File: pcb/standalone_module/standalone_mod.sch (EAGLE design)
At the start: 11 parts, among them U1 V_REG_317DPACK

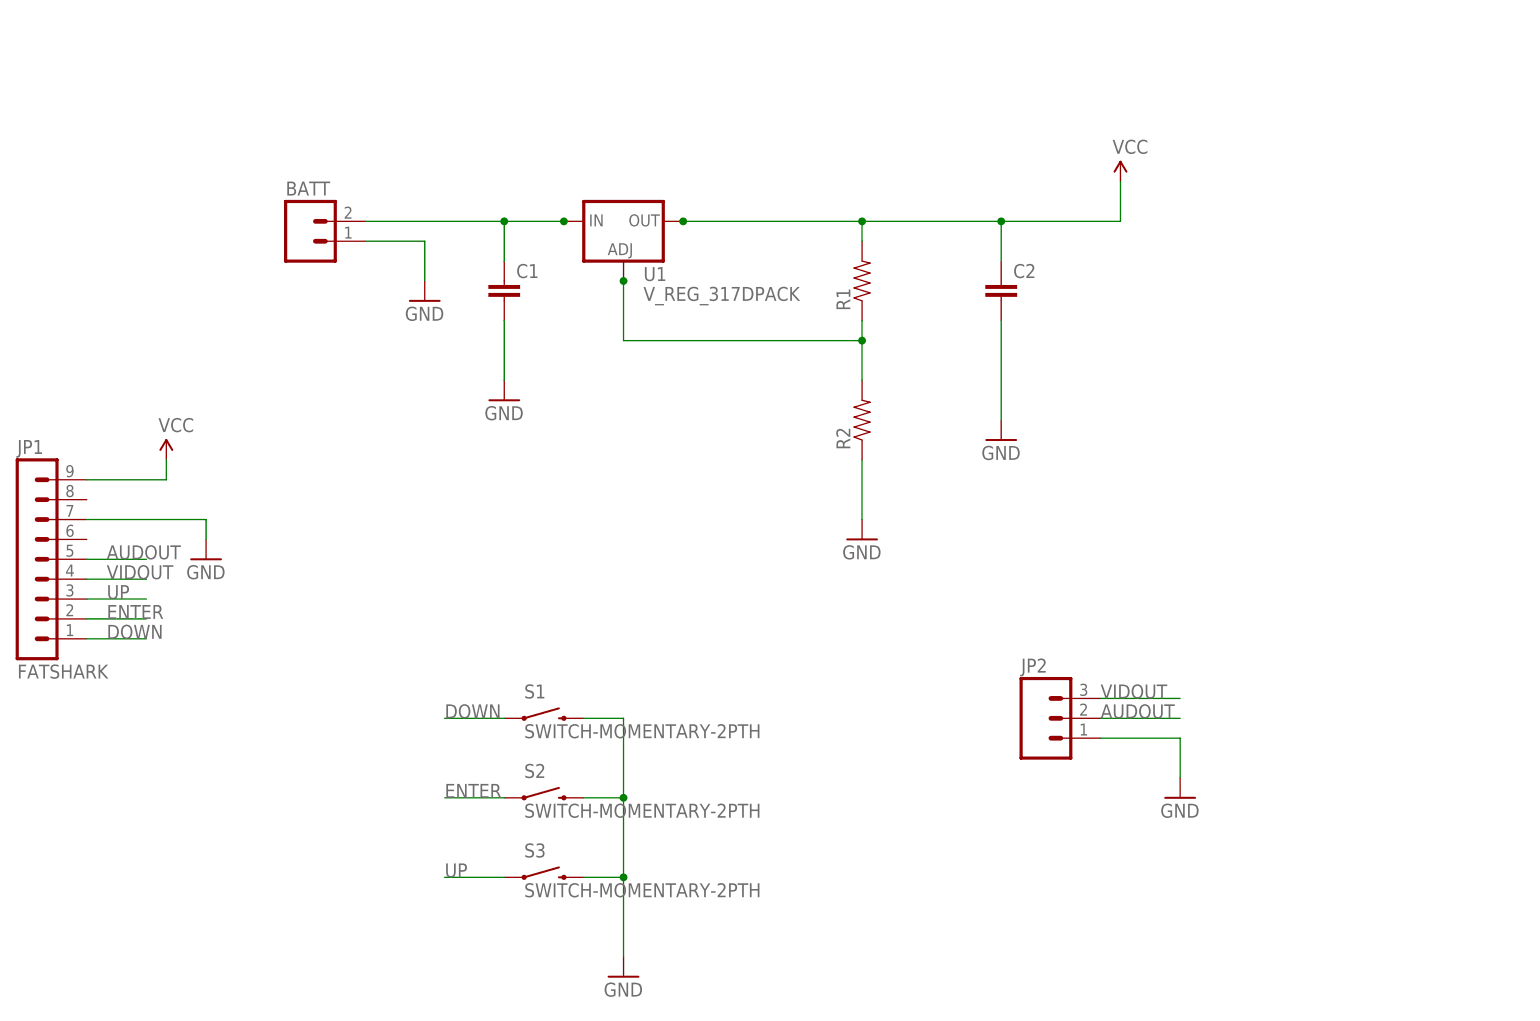
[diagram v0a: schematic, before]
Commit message: standalone v2.0
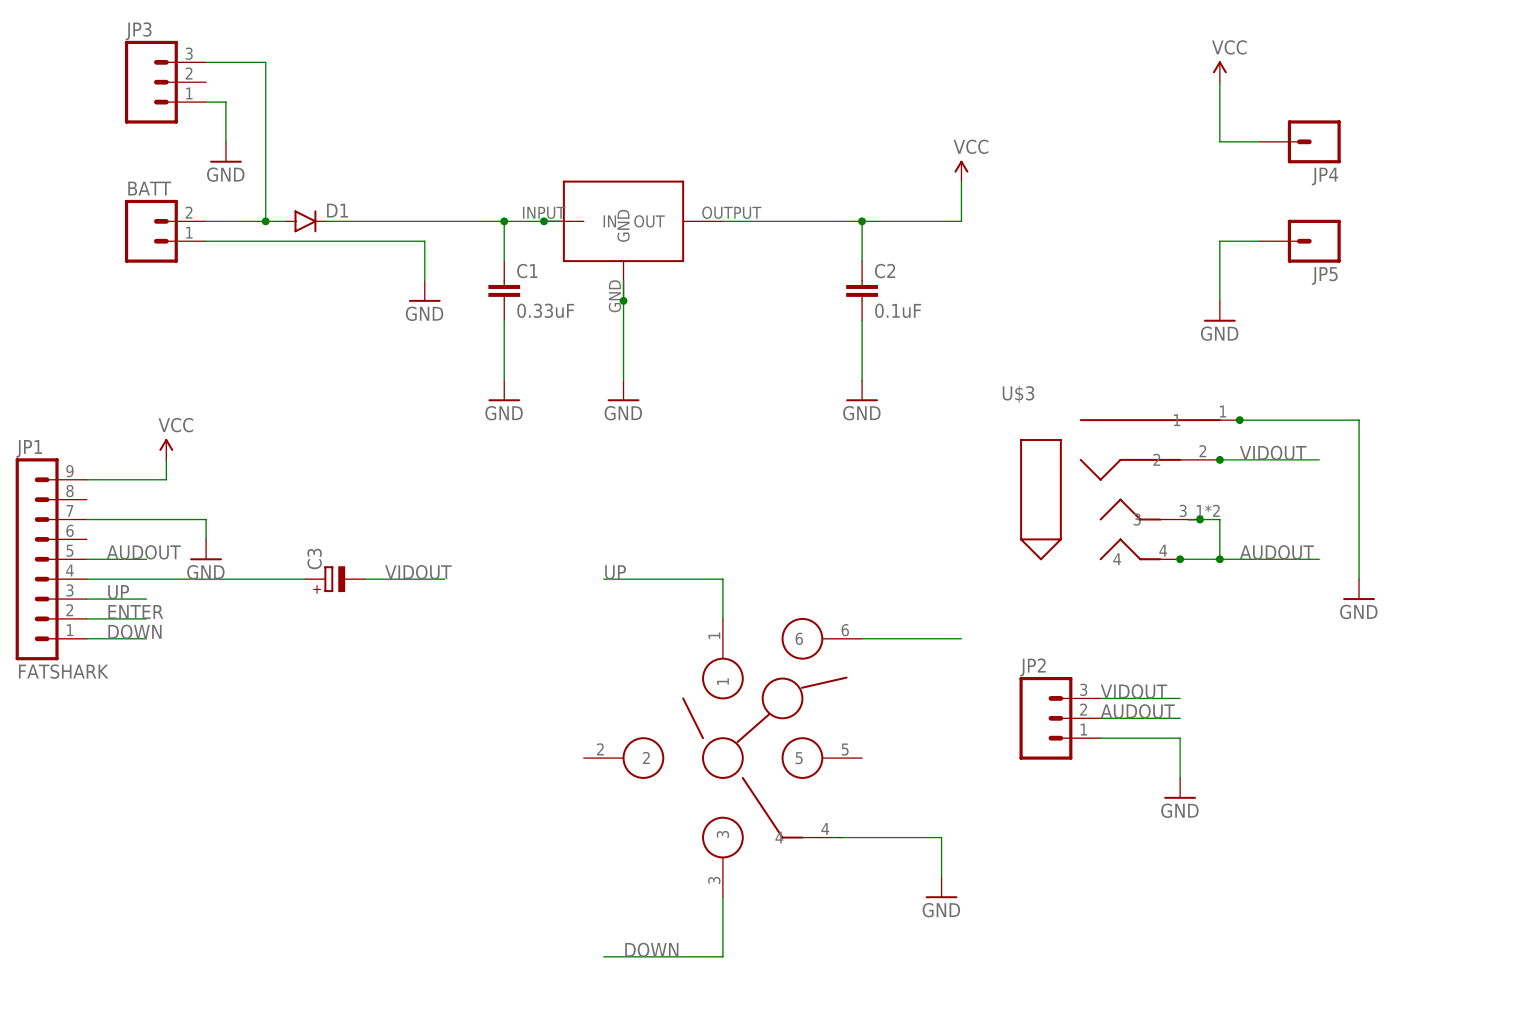
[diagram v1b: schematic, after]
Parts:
- removed R1, R2: (no value), SparkFun-Passives:RESISTOR0805-RES
- removed S1, S2, S3: SWITCH-MOMENTARY-2PTH, SparkFun-Electromechanical:SWITCH-MOMENTARY-2PTH
- removed U1: V_REG_317DPACK, SparkFun-PowerIC:V_REG_317DPACK
- added C3: (no value), resistor:CPOL-EUE3.5-8
- added D1: (no value), SparkFun-DiscreteSemi:DIODESMA
- added JP3: (no value), SparkFun-Connectors:M03LONGPADS
- added JP4, JP5: (no value), SparkFun-Connectors:M01SMD
- added U$1: 7805, #fpv:7805
- added U$2: SKQUCAA010, #fpv:SKQUCAA010
- added U$3: MC001293JACK, #fpv:MC001293JACK
- C1: value (none) -> 0.33uF
- C2: value (none) -> 0.1uF
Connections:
- removed net 3.3V: C2.1, R1.2, U1.OUT
- removed net N$4: R1.1, R2.2, U1.ADJ
- new net N$2: C3.+, JP1.4
- new net N$3: BATT.2, D1.A, JP3.3
- net 5V: now also C2.1, JP4.1, U$1.OUT
- net AUDOUT: now also U$3.3, U$3.4
- net DOWN: now also U$2.3; no longer S1.1
- net ENTER: now also U$2.6; no longer S2.1
- net GND: now also JP3.1, JP5.1, U$1.GND, U$2.4, U$3.1; no longer R2.1, S1.2, S2.2, S3.2
- net N$1: now also D1.C, U$1.IN; no longer BATT.2, U1.IN
- net UP: now also U$2.1; no longer S3.1
- net VIDOUT: now also C3.-, U$3.2; no longer JP1.4
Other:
- moved on the sheet: BATT, C2

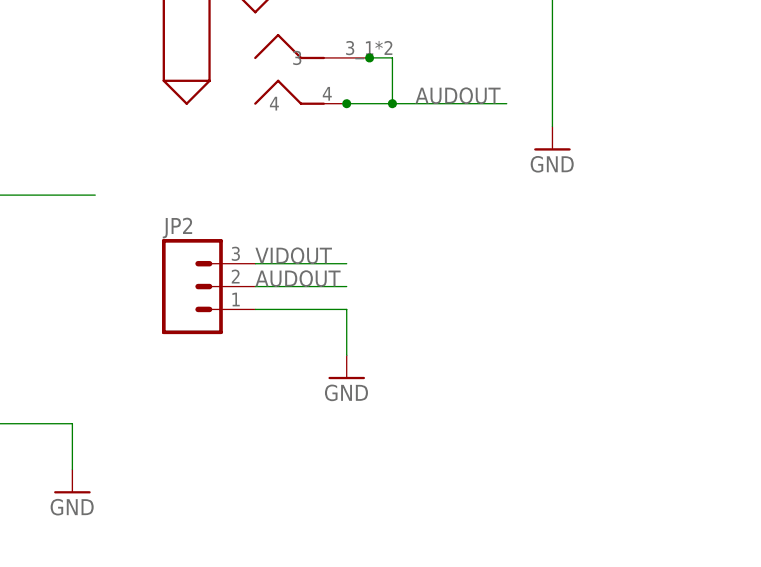
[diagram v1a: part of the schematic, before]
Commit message: standalone module v2
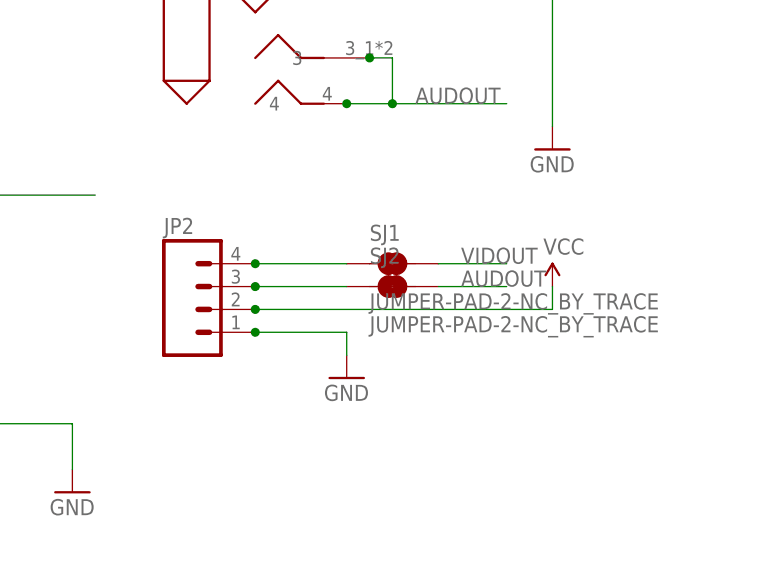
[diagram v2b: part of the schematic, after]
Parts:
- added SJ1, SJ2: JUMPER-PAD-2-NC_BY_TRACE, SparkFun-Passives:JUMPER-PAD-2-NC_BY_TRACE
- JP2: device SparkFun-Connectors:M03PTH -> SparkFun-Connectors:M04PTH
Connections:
- new net N$4: JP2.4, SJ1.1
- new net N$5: JP2.3, SJ2.1
- net 5V: now also JP2.2
- net AUDOUT: now also SJ2.2; no longer JP2.2
- net VIDOUT: now also SJ1.2; no longer JP2.3
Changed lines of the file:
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@@
 <grid distance="0.1" unitdist="inch" unit="inch" style="lines" multiple="1" display="no" altdistance="0.01" altunitdist="inch" altunit="inch"/>
 <layers>
-<layer number="1" name="Top" color="4" fill="1" visible="yes" active="no"/>
-<layer number="16" name="Bottom" color="1" fill="1" visible="yes" active="no"/>
-<layer number="17" name="Pads" color="2" fill="1" visible="yes" active="no"/>
-<layer number="18" name="Vias" color="2" fill="1" visible="yes" active="no"/>
-<layer number="19" name="Unrouted" color="6" fill="1" visible="yes" active="no"/>
-<layer number="20" name="Dimension" color="15" fill="1" visible="yes" active="no"/>
-<layer number="21" name="tPlace" color="7" fill="1" visible="yes" active="no"/>
-<layer number="22" name="bPlace" color="7" fill="1" visible="yes" active="no"/>
-<layer number="23" name="tOrigins" color="15" fill="1" visible="yes" active="no"/>
-<layer number="24" name="bOrigins" color="15" fill="1" visible="yes" active="no"/>
-<layer number="25" name="tNames" color="7" fill="1" visible="yes" active="no"/>
-<layer number="26" name="bNames" color="7" fill="1" visible="yes" active="no"/>
-<layer number="27" name="tValues" color="7" fill="1" visible="yes" active="no"/>
-<layer number="28" name="bValues" color="7" fill="1" visible="yes" active="no"/>
+<layer number="1" name="Top" color="4" fill="1" visible="no" active="no"/>
+<layer number="16" name="Bottom" color="1" fill="1" visible="no" active="no"/>
+<layer number="17" name="Pads" color="2" fill="1" visible="no" active="no"/>
+<layer number="18" name="Vias" color="2" fill="1" visible="no" active="no"/>
+<layer number="19" name="Unrouted" color="6" fill="1" visible="no" active="no"/>
+<layer number="20" name="Dimension" color="15" fill="1" visible="no" active="no"/>
+<layer number="21" name="tPlace" color="7" fill="1" visible="no" active="no"/>
+<layer number="22" name="bPlace" color="7" fill="1" visible="no" active="no"/>
+<layer number="23" name="tOrigins" color="15" fill="1" visible="no" active="no"/>
+<layer number="24" name="bOrigins" color="15" fill="1" visible="no" active="no"/>
+<layer number="25" name="tNames" color="7" fill="1" visible="no" active="no"/>
+<layer number="26" name="bNames" color="7" fill="1" visible="no" active="no"/>
+<layer number="27" name="tValues" color="7" fill="1" visible="no" active="no"/>
+<layer number="28" name="bValues" color="7" fill="1" visible="no" active="no"/>
 <layer number="29" name="tStop" color="7" fill="3" visible="no" active="no"/>
 <layer number="30" name="bStop" color="7" fill="6" visible="no" active="no"/>
@@
 <layer number="35" name="tGlue" color="7" fill="4" visible="no" active="no"/>
 <layer number="36" name="bGlue" color="7" fill="5" visible="no" active="no"/>
-<layer number="37" name="tTest" color="7" fill="1" visible="yes" active="no"/>
-<layer number="38" name="bTest" color="7" fill="1" visible="yes" active="no"/>
+<layer number="37" name="tTest" color="7" fill="1" visible="no" active="no"/>
+<layer number="38" name="bTest" color="7" fill="1" visible="no" active="no"/>
 <layer number="39" name="tKeepout" color="4" fill="11" visible="no" active="no"/>
 <layer number="40" name="bKeepout" color="1" fill="11" visible="no" active="no"/>
@@
 <layer number="44" name="Drills" color="7" fill="1" visible="no" active="no"/>
 <layer number="45" name="Holes" color="7" fill="1" visible="no" active="no"/>
-<layer number="46" name="Milling" color="3" fill="1" visible="yes" active="no"/>
-<layer number="47" name="Measures" color="7" fill="1" visible="yes" active="no"/>
-<layer number="48" name="Document" color="7" fill="1" visible="yes" active="no"/>
-<layer number="49" name="Reference" color="7" fill="1" visible="yes" active="no"/>
-<layer number="50" name="dxf" color="7" fill="1" visible="yes" active="no"/>
-<layer number="51" name="tDocu" color="7" fill="1" visible="yes" active="no"/>
-<layer number="52" name="bDocu" color="7" fill="1" visible="yes" active="no"/>
-<layer number="53" name="tGND_GNDA" color="7" fill="1" visible="yes" active="no"/>
-<layer number="54" name="bGND_GNDA" color="7" fill="1" visible="yes" active="no"/>
-<layer number="56" name="wert" color="7" fill="1" visible="yes" active="no"/>
-<layer number="57" name="tCAD" color="7" fill="1" visible="yes" active="no"/>
-<layer number="59" name="tCarbon" color="7" fill="1" visible="yes" active="no"/>
-<layer number="60" name="bCarbon" color="7" fill="1" visible="yes" active="no"/>
+<layer number="46" name="Milling" color="3" fill="1" visible="no" active="no"/>
+<layer number="47" name="Measures" color="7" fill="1" visible="no" active="no"/>
+<layer number="48" name="Document" color="7" fill="1" visible="no" active="no"/>
+<layer number="49" name="Reference" color="7" fill="1" visible="no" active="no"/>
+<layer number="50" name="dxf" color="7" fill="1" visible="no" active="no"/>
+<layer number="51" name="tDocu" color="7" fill="1" visible="no" active="no"/>
+<layer number="52" name="bDocu" color="7" fill="1" visible="no" active="no"/>
+<layer number="53" name="tGND_GNDA" color="7" fill="1" visible="no" active="no"/>
+<layer number="54" name="bGND_GNDA" color="7" fill="1" visible="no" active="no"/>
+<layer number="56" name="wert" color="7" fill="1" visible="no" active="no"/>
+<layer number="57" name="tCAD" color="7" fill="1" visible="no" active="no"/>
+<layer number="59" name="tCarbon" color="7" fill="1" visible="no" active="no"/>
+<layer number="60" name="bCarbon" color="7" fill="1" visible="no" active="no"/>
 <layer number="90" name="Modules" color="5" fill="1" visible="yes" active="yes"/>
 <layer number="91" name="Nets" color="2" fill="1" visible="yes" active="yes"/>
@@
 <part name="P+1" library="SparkFun" deviceset="3.3V" device="" value="VCC"/>
 <part name="GND4" library="supply1" deviceset="GND" device=""/>
-<part name="JP2" library="SparkFun-Connectors" deviceset="M03" device="PTH"/>
 <part name="GND6" library="supply1" deviceset="GND" device=""/>
 <part name="U$1" library="#fpv" deviceset="7805" device=""/>
@@
 <part name="P+2" library="SparkFun" deviceset="3.3V" device="" value="VCC"/>
 <part name="GND9" library="supply1" deviceset="GND" device=""/>
+<part name="JP2" library="SparkFun-Connectors" deviceset="M04" device="PTH"/>
+<part name="P+4" library="SparkFun" deviceset="3.3V" device="" value="VCC"/>
+<part name="SJ1" library="SparkFun-Passives" deviceset="JUMPER-PAD-2-NC_BY_TRACE" device=""/>
+<part name="SJ2" library="SparkFun-Passives" deviceset="JUMPER-PAD-2-NC_BY_TRACE" device=""/>
 </parts>
 <sheets>
@@
 <instance part="P+1" gate="G$1" x="165.1" y="170.18"/>
 <instance part="GND4" gate="1" x="96.52" y="154.94"/>
-<instance part="JP2" gate="G$1" x="175.26" y="101.6"/>
 <instance part="GND6" gate="1" x="193.04" y="91.44"/>
 <instance part="U$1" gate="G$1" x="121.92" y="160.02"/>
@@
 <instance part="P+2" gate="G$1" x="198.12" y="182.88"/>
 <instance part="GND9" gate="1" x="198.12" y="152.4"/>
+<instance part="JP2" gate="G$1" x="177.8" y="99.06"/>
+<instance part="P+4" gate="G$1" x="215.9" y="101.6"/>
+<instance part="SJ1" gate="G$1" x="198.12" y="104.14"/>
+<instance part="SJ2" gate="G$1" x="198.12" y="101.6"/>
 </instances>
 <busses>
@@
 </segment>
 <segment>
+<wire x1="193.04" y1="96.52" x2="193.04" y2="93.98" width="0.1524" layer="91"/>
+<pinref part="GND6" gate="1" pin="GND"/>
 <pinref part="JP2" gate="G$1" pin="1"/>
-<wire x1="182.88" y1="99.06" x2="193.04" y2="99.06" width="0.1524" layer="91"/>
-<wire x1="193.04" y1="99.06" x2="193.04" y2="93.98" width="0.1524" layer="91"/>
-<pinref part="GND6" gate="1" pin="GND"/>
+<wire x1="193.04" y1="96.52" x2="182.88" y2="96.52" width="0.1524" layer="91"/>
+<junction x="182.88" y="96.52"/>
 </segment>
 <segment>
@@
 <pinref part="P+2" gate="G$1" pin="3.3V"/>
 </segment>
+<segment>
+<pinref part="JP2" gate="G$1" pin="2"/>
+<wire x1="182.88" y1="99.06" x2="215.9" y2="99.06" width="0.1524" layer="91"/>
+<wire x1="215.9" y1="99.06" x2="215.9" y2="101.6" width="0.1524" layer="91"/>
+<pinref part="P+4" gate="G$1" pin="3.3V"/>
+<junction x="182.88" y="99.06"/>
+</segment>
 </net>
 <net name="VIDOUT" class="0">
-<segment>
-<pinref part="JP2" gate="G$1" pin="3"/>
-<wire x1="182.88" y1="104.14" x2="193.04" y2="104.14" width="0.1524" layer="91"/>
-<label x="182.88" y="104.14" size="1.778" layer="95"/>
-</segment>
 <segment>
 <pinref part="C3" gate="G$1" pin="-"/>
@@
 <junction x="198.12" y="134.62"/>
 </segment>
+<segment>
+<pinref part="SJ1" gate="G$1" pin="2"/>
+<wire x1="203.2" y1="104.14" x2="210.82" y2="104.14" width="0.1524" layer="91"/>
+<label x="205.74" y="104.14" size="1.778" layer="95"/>
+</segment>
 </net>
 <net name="AUDOUT" class="0">
@@
 <wire x1="53.34" y1="121.92" x2="60.96" y2="121.92" width="0.1524" layer="91"/>
 <label x="55.88" y="121.92" size="1.778" layer="95"/>
-</segment>
-<segment>
-<pinref part="JP2" gate="G$1" pin="2"/>
-<wire x1="182.88" y1="101.6" x2="193.04" y2="101.6" width="0.1524" layer="91"/>
-<label x="182.88" y="101.6" size="1.778" layer="95"/>
 </segment>
 <segment>
@@
 <junction x="193.04" y="121.92"/>
 </segment>
+<segment>
+<pinref part="SJ2" gate="G$1" pin="2"/>
+<wire x1="203.2" y1="101.6" x2="210.82" y2="101.6" width="0.1524" layer="91"/>
+<label x="205.74" y="101.6" size="1.778" layer="95"/>
+</segment>
 </net>
 <net name="N$1" class="0">
@@
 </segment>
 </net>
+<net name="N$4" class="0">
+<segment>
+<pinref part="SJ1" gate="G$1" pin="1"/>
+<pinref part="JP2" gate="G$1" pin="4"/>
+<wire x1="193.04" y1="104.14" x2="182.88" y2="104.14" width="0.1524" layer="91"/>
+<junction x="182.88" y="104.14"/>
+</segment>
+</net>
+<net name="N$5" class="0">
+<segment>
+<pinref part="SJ2" gate="G$1" pin="1"/>
+<pinref part="JP2" gate="G$1" pin="3"/>
+<wire x1="193.04" y1="101.6" x2="182.88" y2="101.6" width="0.1524" layer="91"/>
+<junction x="182.88" y="101.6"/>
+</segment>
+</net>
